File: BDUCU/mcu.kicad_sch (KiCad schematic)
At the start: 15 parts, among them SW1 SW_Push, U8 ATmega328-A, Y1 16MHz

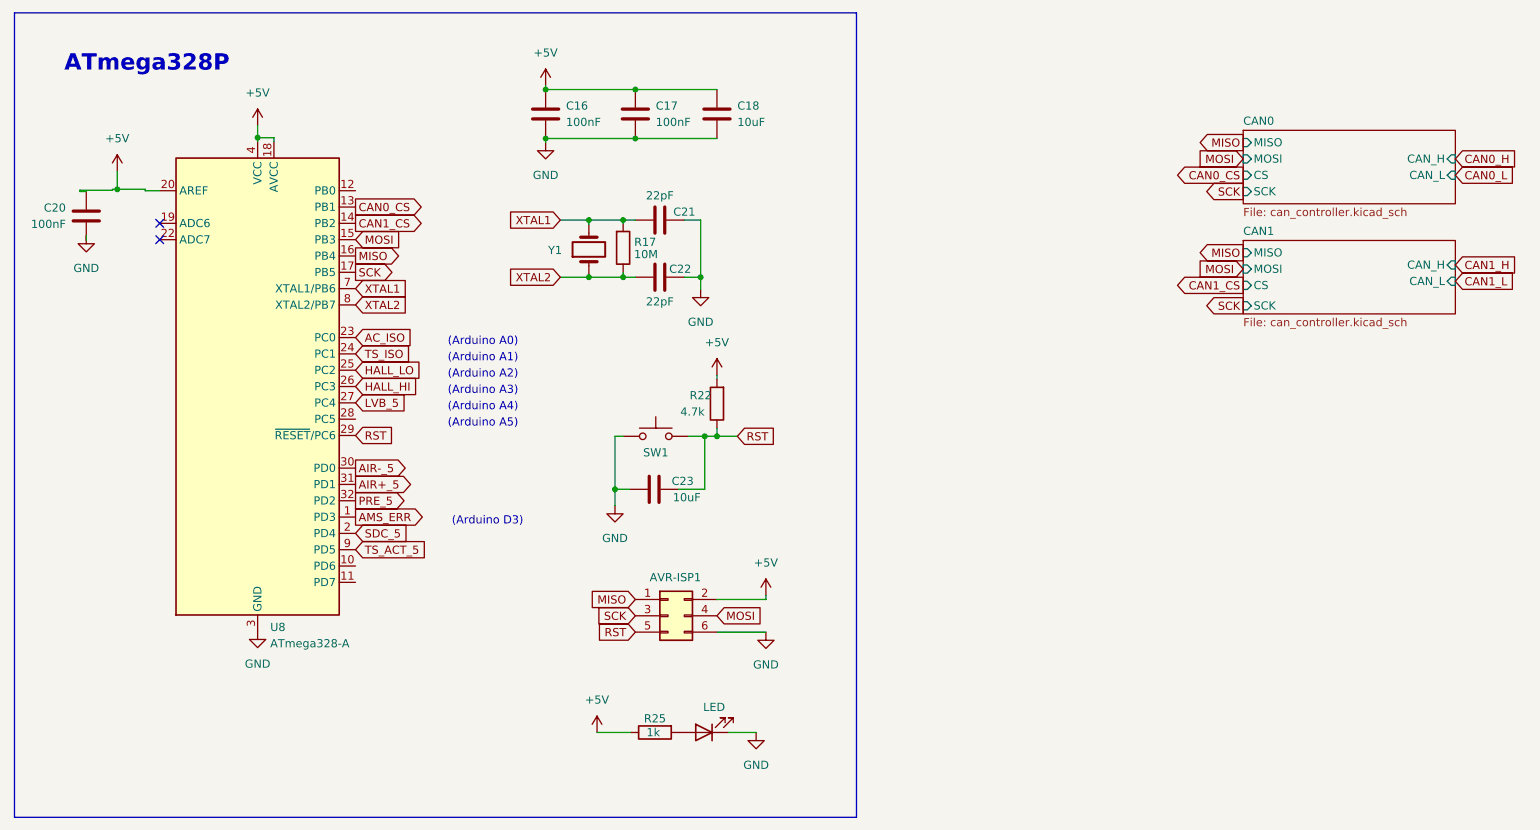
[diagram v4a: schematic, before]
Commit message: Finished BDUCU layout, silkscreen remaining
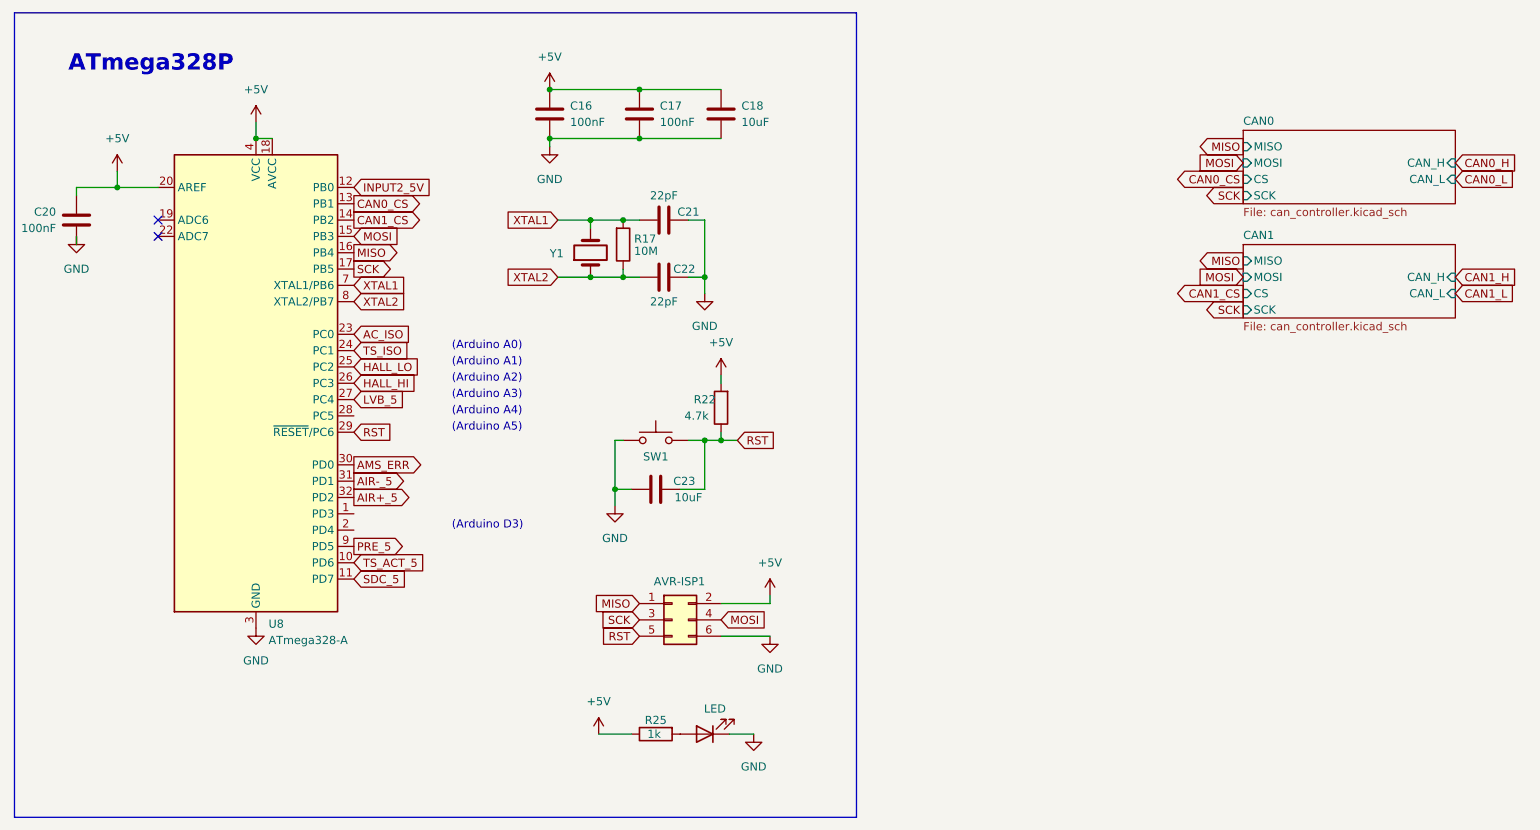
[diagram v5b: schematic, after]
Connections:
- net AIR+_5: now also U8.32 (PD2); no longer U8.31 (PD1)
- net AIR-_5: now also U8.31 (PD1); no longer U8.30 (PD0)
- net AMS_ERR: now also U8.30 (PD0); no longer U8.1 (PD3)
- net PRE_5: now also U8.9 (PD5); no longer U8.32 (PD2)
- net SDC_5: now also U8.11 (PD7); no longer U8.2 (PD4)
- net TS_ACT_5: now also U8.10 (PD6); no longer U8.9 (PD5)
- net INPUT2_5V: now reaches U8.12 (PB0)
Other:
- moved on the sheet: AVR-ISP1, C16, C17, C18, C20, C21, C22, R17, R22, SW1, U8, Y1
